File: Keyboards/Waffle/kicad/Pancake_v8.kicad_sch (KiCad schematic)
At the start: 91 parts, among them J10 TC2030_SWD, J2 HRO_TYPE-C-31-M-14, J3 Battery, Q2 2N7002, SW1 PWR, SW1 SW_Push_45deg, SW10 SW_Push_45deg, SW11 SW_Push_45deg, SW12 SW_Push_45deg, SW13 SW_Push_45deg, SW14 SW_Push_45deg, SW15 SW_Push_45deg, SW16 SW_Push_45deg, SW17 SW_Push_45deg, SW18 SW_Push_45deg, SW19 SW_Push_45deg, SW2 SW_Push_45deg, SW20 SW_Push_45deg, SW21 SW_Push_45deg, SW22 SW_Push_45deg, SW23 SW_Push_45deg, SW24 SW_Push_45deg, SW25 SW_Push_45deg, SW26 SW_Push_45deg, SW3 SW_Push_45deg, SW4 SW_Push_45deg, SW5 RST, SW5 SW_Push_45deg, SW6 SW_Push_45deg, SW7 SW_Push_45deg, SW8 SW_Push_45deg, SW9 SW_Push_45deg, U1 SRV05-4, U3 BQ24075, U9 nRF52840_E73-2G4M08S1C, Y1 32.768 KHz

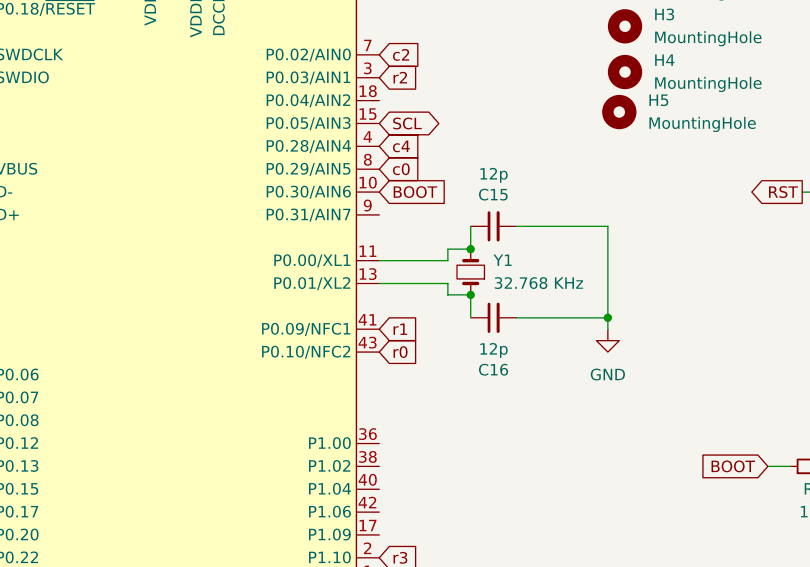
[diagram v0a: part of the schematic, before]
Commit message: Update waffle proto
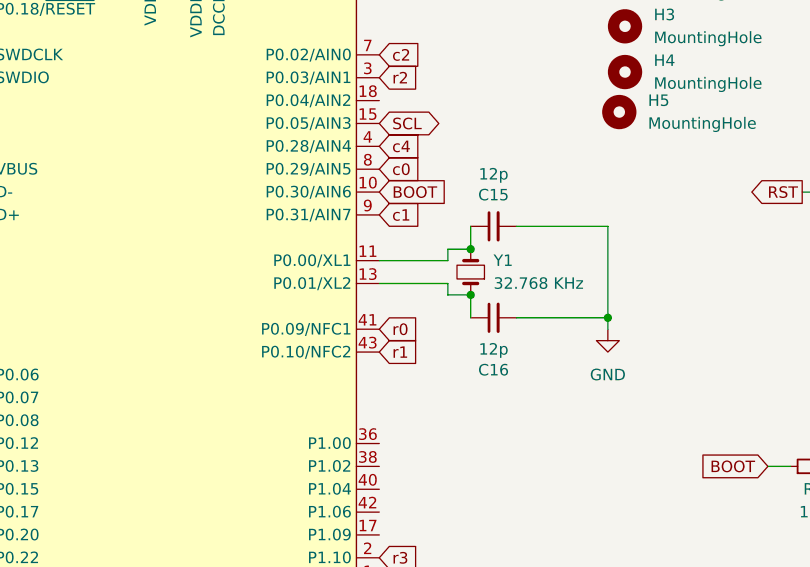
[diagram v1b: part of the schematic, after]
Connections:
- net c1: now also U9.9 (P0.31/AIN7)
- net r0: now also U9.41 (P0.09/NFC1); no longer U9.43 (P0.10/NFC2)
- net r1: now also U9.43 (P0.10/NFC2); no longer U9.41 (P0.09/NFC1)
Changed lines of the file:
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@@
 	(global_label "r1"
 		(shape input)
-		(at 153.67 134.62 0)
-		(fields_autoplaced yes)
-		(effects
-			(font
-				(size 1.27 1.27)
-			)
-			(justify left)
-		)
-		(property "Intersheetrefs" "${INTERSHEET_REFS}"
-			(at 158.6509 134.62 0)
+		(at 153.67 137.16 0)
+		(fields_autoplaced yes)
+		(effects
+			(font
+				(size 1.27 1.27)
+			)
+			(justify left)
+		)
+		(property "Intersheetrefs" "${INTERSHEET_REFS}"
+			(at 158.6509 137.16 0)
 			(effects
 				(font
@@
 		)
 	)
+	(global_label "c1"
+		(shape input)
+		(at 153.67 121.92 0)
+		(fields_autoplaced yes)
+		(effects
+			(font
+				(size 1.27 1.27)
+			)
+			(justify left)
+		)
+		(property "Intersheetrefs" "${INTERSHEET_REFS}"
+			(at 158.9533 121.92 0)
+			(effects
+				(font
+					(size 1.27 1.27)
+				)
+				(justify left)
+				(hide yes)
+			)
+		)
+	)
 	(global_label "USB-D-"
 		(shape bidirectional)
@@
 				)
 				(justify right)
+				(hide yes)
+			)
+		)
+	)
+	(global_label "r0"
+		(shape input)
+		(at 153.67 134.62 0)
+		(fields_autoplaced yes)
+		(effects
+			(font
+				(size 1.27 1.27)
+			)
+			(justify left)
+		)
+		(property "Intersheetrefs" "${INTERSHEET_REFS}"
+			(at 158.6509 134.62 0)
+			(effects
+				(font
+					(size 1.27 1.27)
+				)
+				(justify left)
 				(hide yes)
 			)
@@
 				(hide yes)
 			)
-		)
-	)
-	(global_label "r0"
-		(shape input)
-		(at 153.67 137.16 0)
-		(fields_autoplaced yes)
-		(effects
-			(font
-				(size 1.27 1.27)
-			)
-			(justify left)
-		)
-		(property "Intersheetrefs" "${INTERSHEET_REFS}"
-			(at 158.6509 137.16 0)
-			(effects
-				(font
-					(size 1.27 1.27)
-				)
-				(justify left)
-				(hide yes)
-			)
